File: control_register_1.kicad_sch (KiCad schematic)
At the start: 6 parts, among them U10 74HC375, U11 74HC02, U12 74HC21, U13 74HC21, U7 74HC04, U9 74HC375

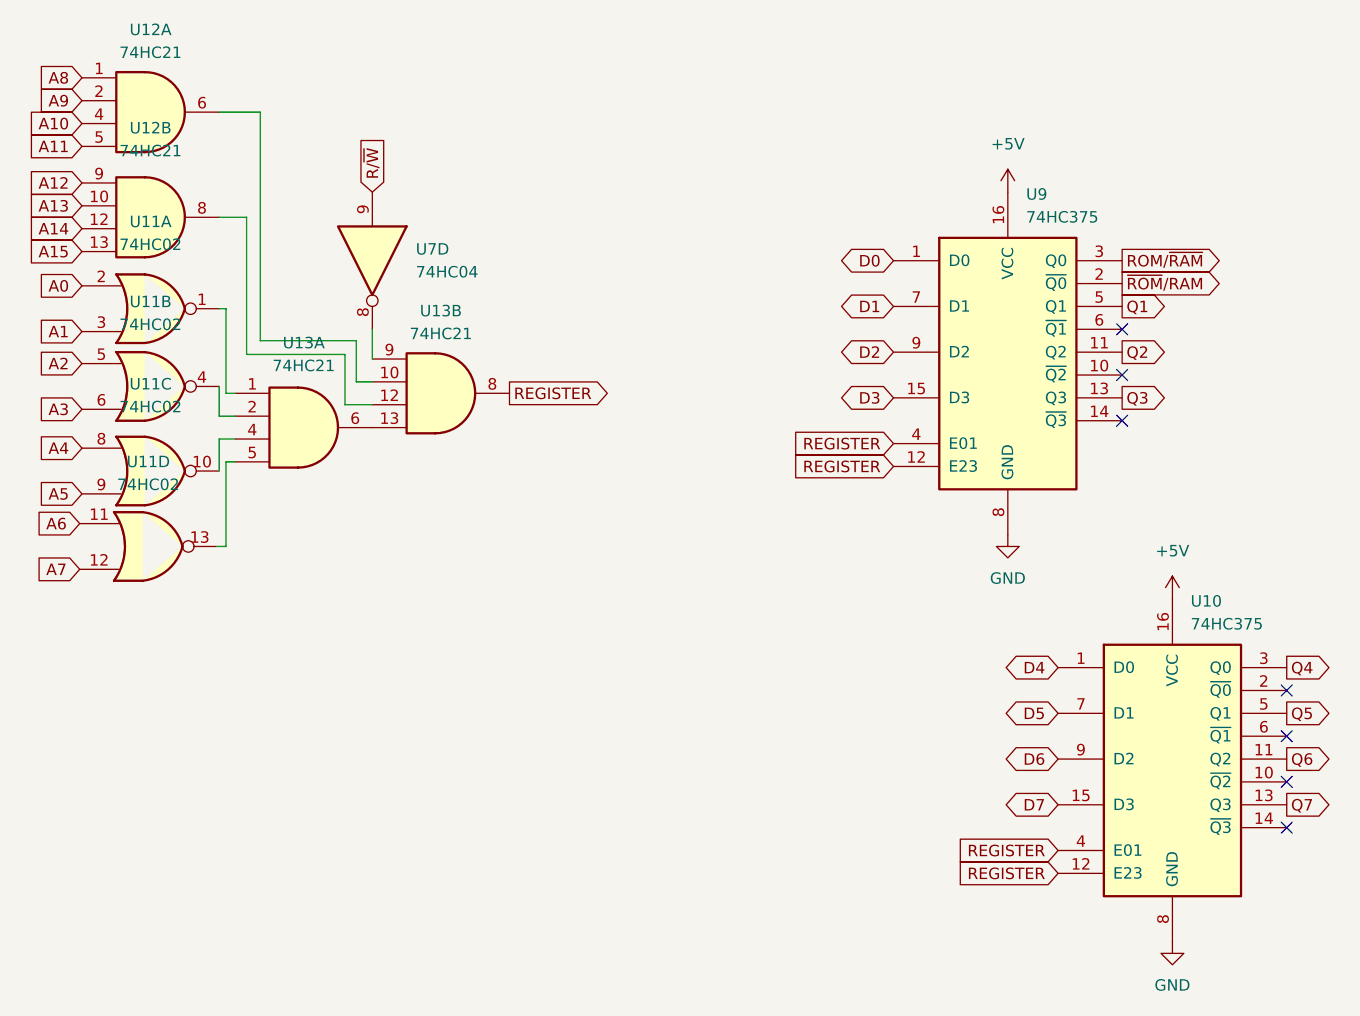
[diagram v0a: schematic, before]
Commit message: rearrange components for routing
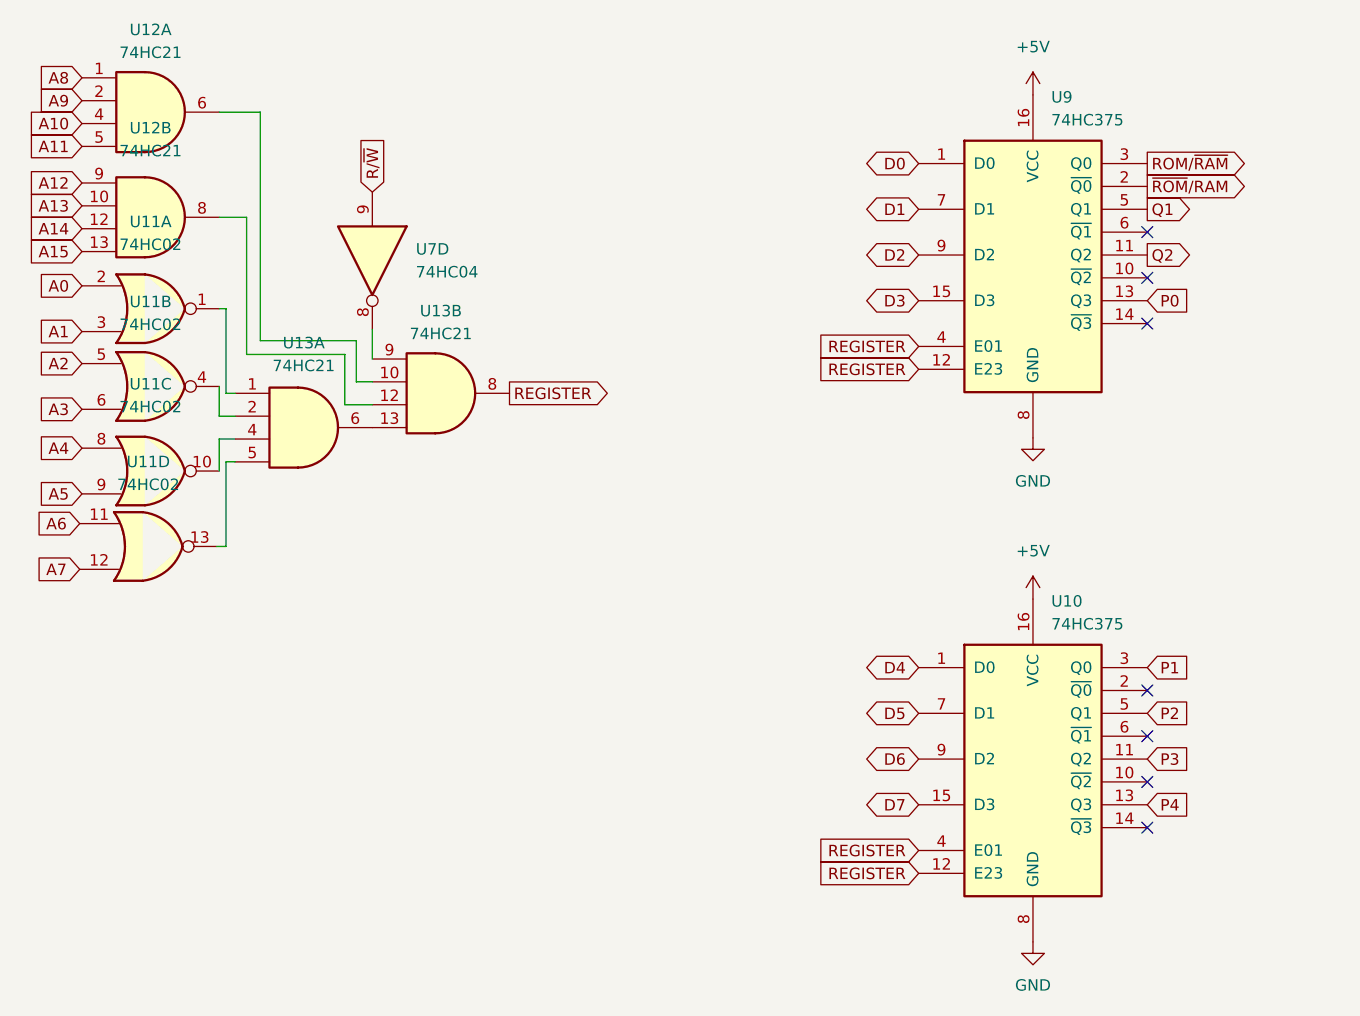
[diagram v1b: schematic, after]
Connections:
- net Q3 renamed P0
- net Q4 renamed P1
- net Q5 renamed P2
- net Q6 renamed P3
- net Q7 renamed P4
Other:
- moved on the sheet: U10, U9
